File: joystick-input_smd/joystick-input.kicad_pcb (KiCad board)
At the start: 2 copper layers, 53.3 x 29.5 mm, 19 parts, among them J1 Conn_01x18, J2 Conn_02x14_Odd_Even

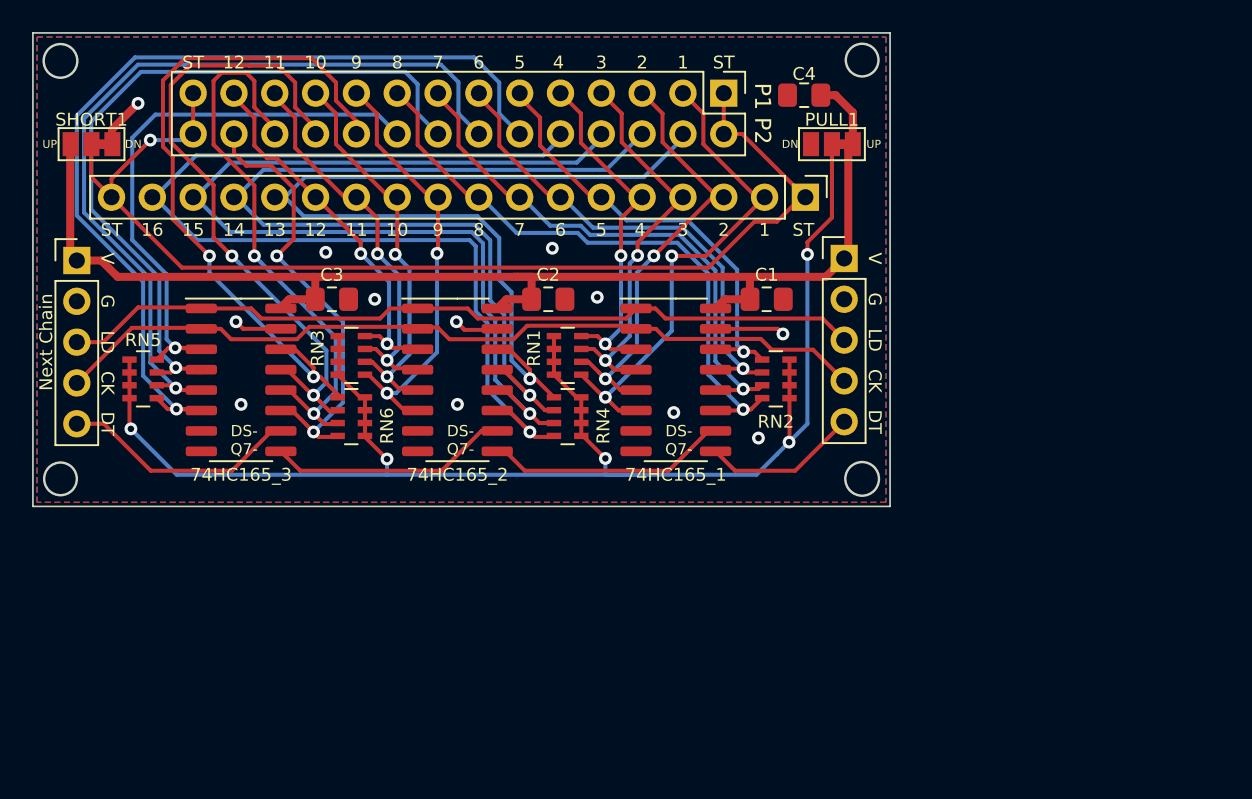
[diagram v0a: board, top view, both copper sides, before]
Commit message: 도면 시트 설명 추가
Signed-off-by: Ju, Gyeong-min <jcmh74@gmail.com>
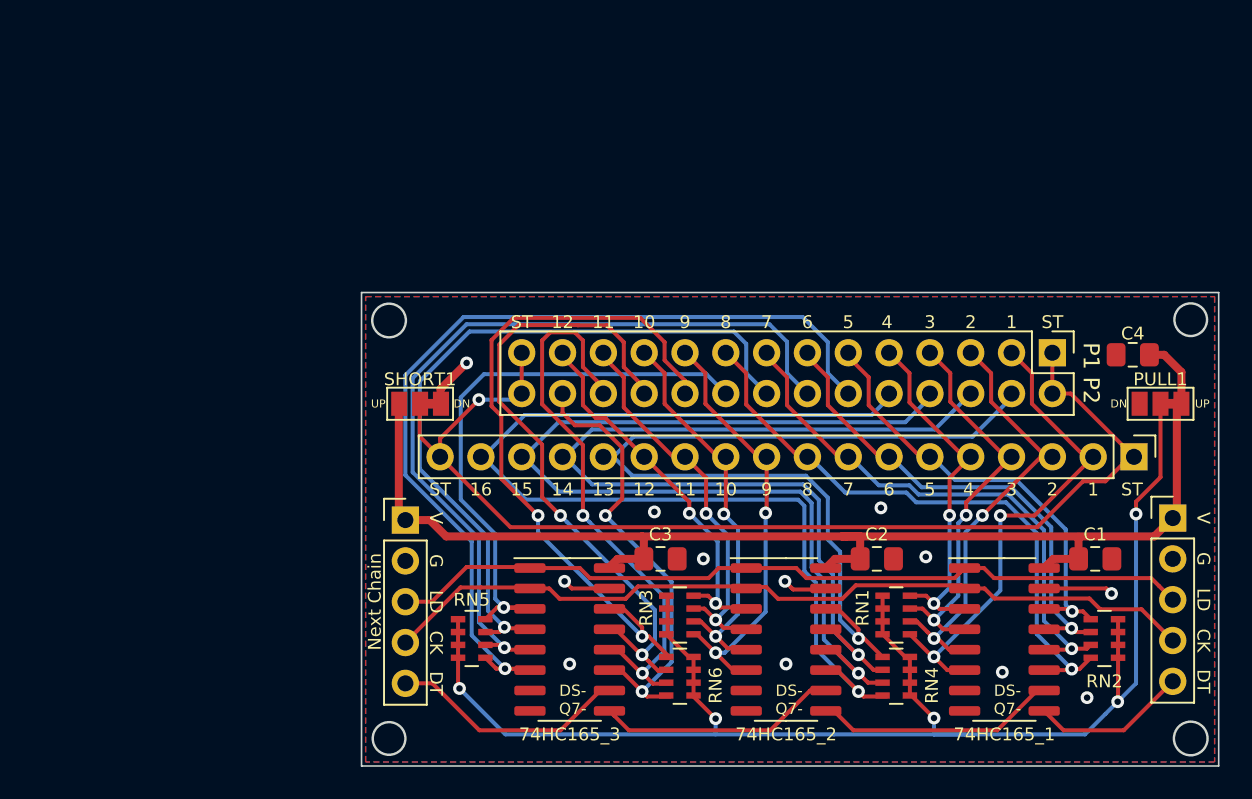
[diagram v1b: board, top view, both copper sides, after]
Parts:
- moved 74HC165_1 26.1 mm to (172.3, 105.5)
- moved 74HC165_2 26.1 mm to (158.7, 105.5)
- moved 74HC165_3 26.1 mm to (145.2, 105.5)
- moved J1 26.1 mm to (180.3, 94.1)
- moved RN1 26.1 mm to (165.5, 104.0)
- moved RN3 26.1 mm to (152.1, 104.0)
- moved C1 26.1 mm to (177.9, 100.5)
- moved C2 26.1 mm to (164.3, 100.5)
- moved C3 26.1 mm to (150.9, 100.5)
- moved C4 26.1 mm to (180.3, 87.8)
- moved IN1 26.1 mm to (135.0, 98.1)
- moved J2 26.1 mm to (175.3, 87.7)
- moved PULL1 26.1 mm to (182.0, 90.8)
- moved RN2 26.1 mm to (178.5, 105.4)
- moved RN4 26.1 mm to (165.5, 107.8)
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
